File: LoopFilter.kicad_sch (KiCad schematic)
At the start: 13 parts, among them IC1 RRA78610-QAJ

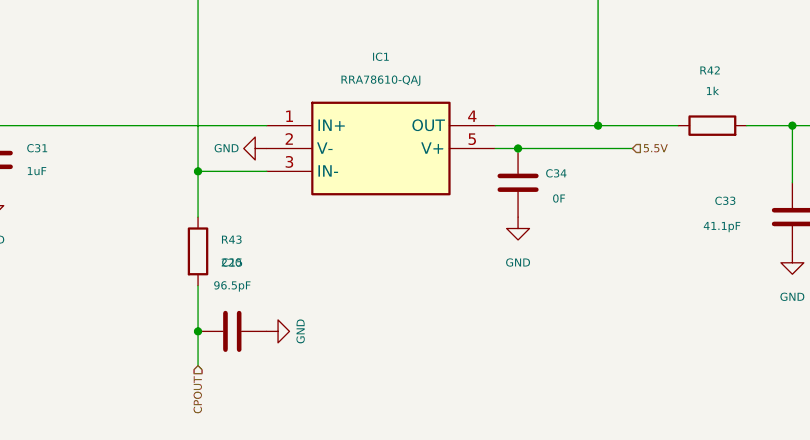
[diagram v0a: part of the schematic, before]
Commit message: complete pcb design
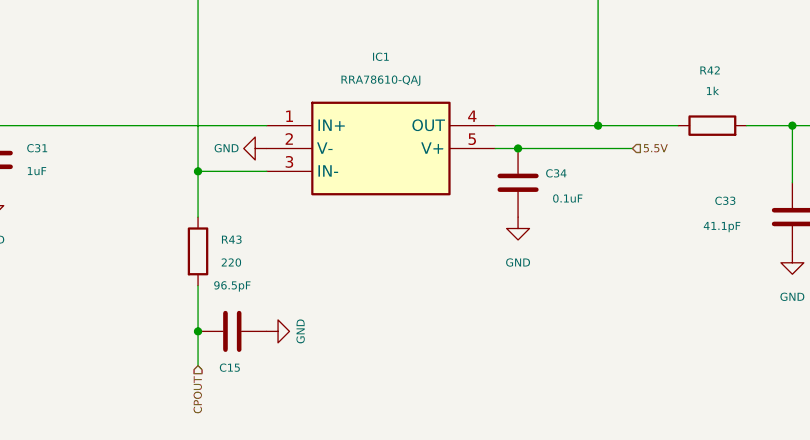
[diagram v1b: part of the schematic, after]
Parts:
- C34: value 0F -> 0.1uF
- R39: footprint Resistor_SMD:R_0603_1608Metric -> Resistor_SMD:R_0402_1005Metric
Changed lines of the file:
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@@
 			)
 		)
-		(property "Value" "0F"
+		(property "Value" "0.1uF"
 			(at 135.89 83.058 0)
 			(show_name no)
@@
 		(in_pos_files yes)
 		(dnp no)
-		(fields_autoplaced yes)
 		(property "Reference" "C15"
-			(at 100.33 90.17 90)
+			(at 100.076 101.854 90)
 			(show_name no)
 			(do_not_autoplace no)
@@
 			)
 		)
-		(property "Footprint" "Resistor_SMD:R_0603_1608Metric"
+		(property "Footprint" "Resistor_SMD:R_0402_1005Metric"
 			(at 56.642 69.85 90)
 			(hide yes)
